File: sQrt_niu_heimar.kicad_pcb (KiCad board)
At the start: 2 copper layers, 84 x 100 mm, 130 parts, among them J1 NMJ6HCD2, J2 NMJ6HCD2, J3 MJ-179PH, Q1 2SC2240, Q2 2SK303, Q3 2SK303, SW1 SW_SPST, U1 TL074, U2 TL074, U4 MC34063AP, U5 TL072, U6 NJM2397, U7 4013

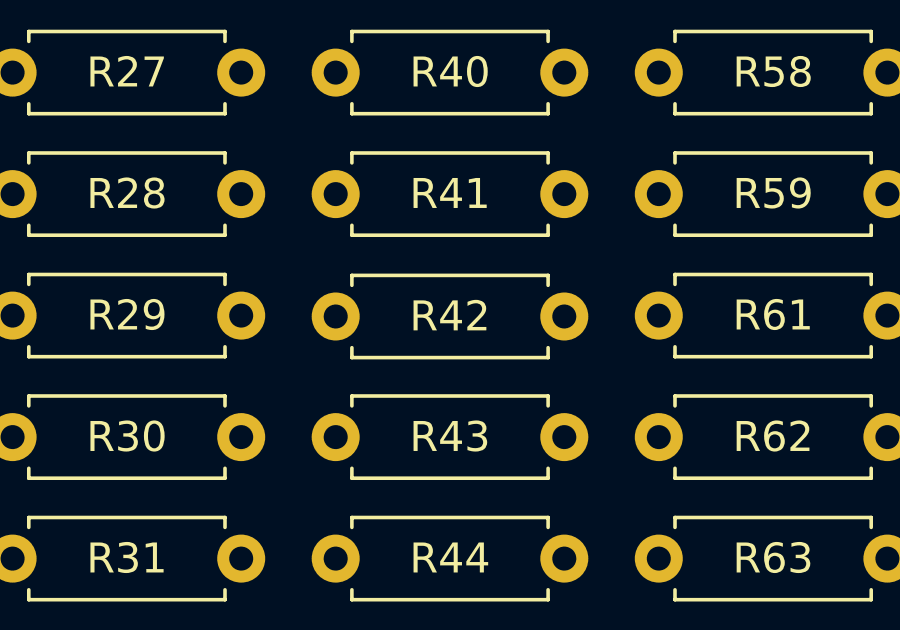
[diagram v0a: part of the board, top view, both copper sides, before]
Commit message: v1.0.1_test
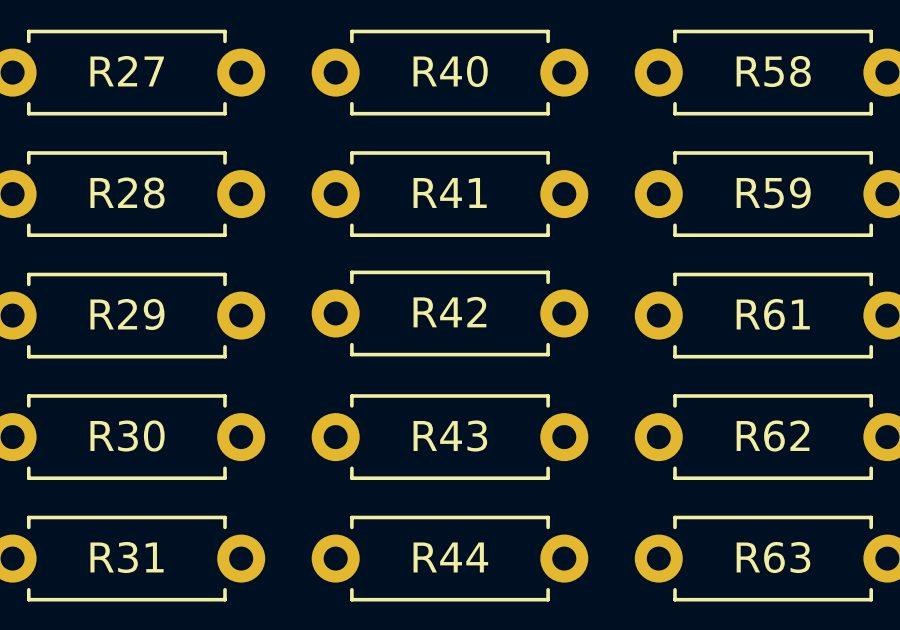
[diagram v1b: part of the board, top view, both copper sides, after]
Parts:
- moved R42 0.10 mm to (229.0, 42.5)
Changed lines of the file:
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@@
   )
   (footprint "Resistor_THT:R_Axial_DIN0207_L6.3mm_D2.5mm_P7.62mm_Horizontal" (layer "F.Cu")
-    (at 228.97 42.6)
+    (at 228.97 42.5)
     (descr "Resistor, Axial_DIN0207 series, Axial, Horizontal, pin pitch=7.62mm, 0.25W = 1/4W, length*diameter=6.3*2.5mm^2, http://cdn-reichelt.de/documents/datenblatt/B400/1_4W%23YAG.pdf")
     (tags "Resistor Axial_DIN0207 series Axial Horizontal pin pitch 7.62mm 0.25W = 1/4W length 6.3mm diameter 2.5mm")
